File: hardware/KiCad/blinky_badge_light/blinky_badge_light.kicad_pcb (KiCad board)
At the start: 4 copper layers, 108.6 x 87.8 mm, 120 parts, among them Q1 N-Channel MOSFET, Q2 Q_PMOS_GSD, Q3 N-Channel MOSFET, SW1 TS-1187A-B-A-B, U1 ESP32-S3-WROOM-1, U2 TP4056, U3 AP2112K-3.3, U4 MT3608, U5 CP2102N-Axx-xQFN24, U6 SN74LVC1T45DBV

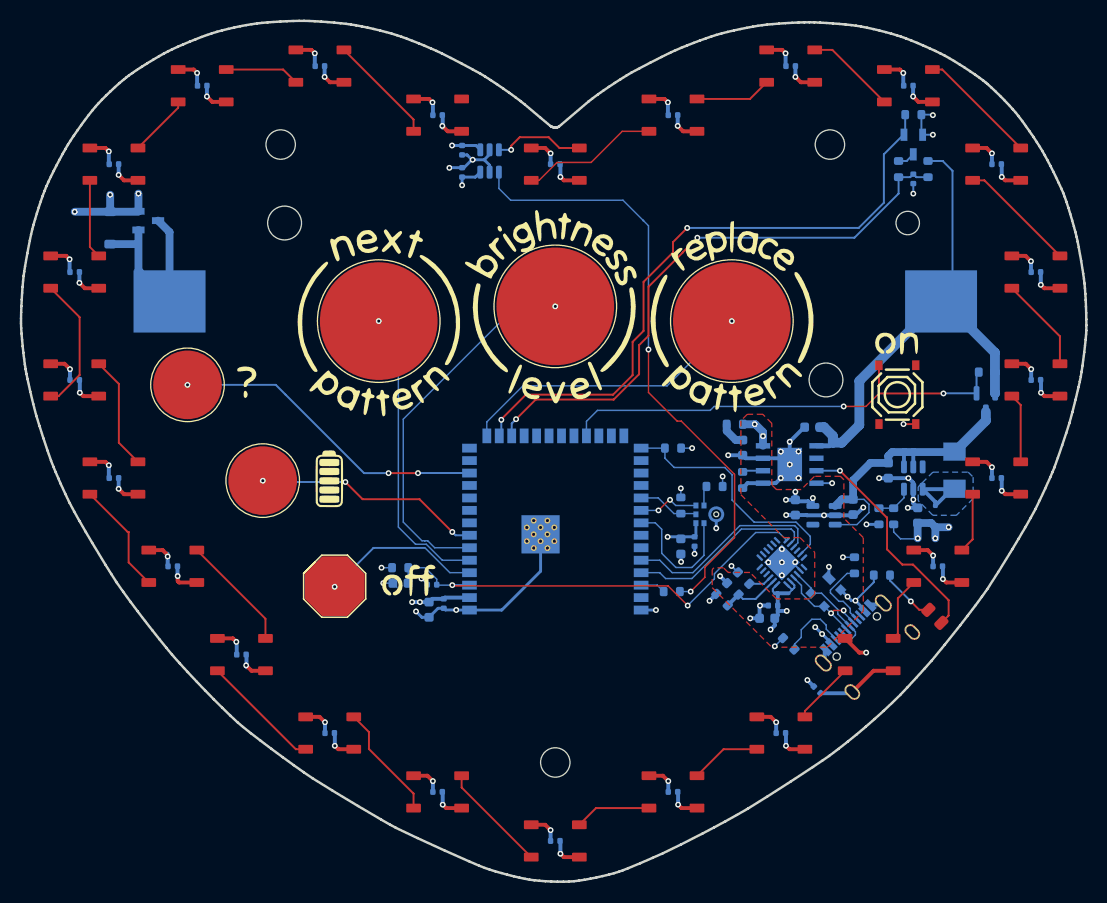
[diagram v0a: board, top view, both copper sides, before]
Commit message: hanger ring
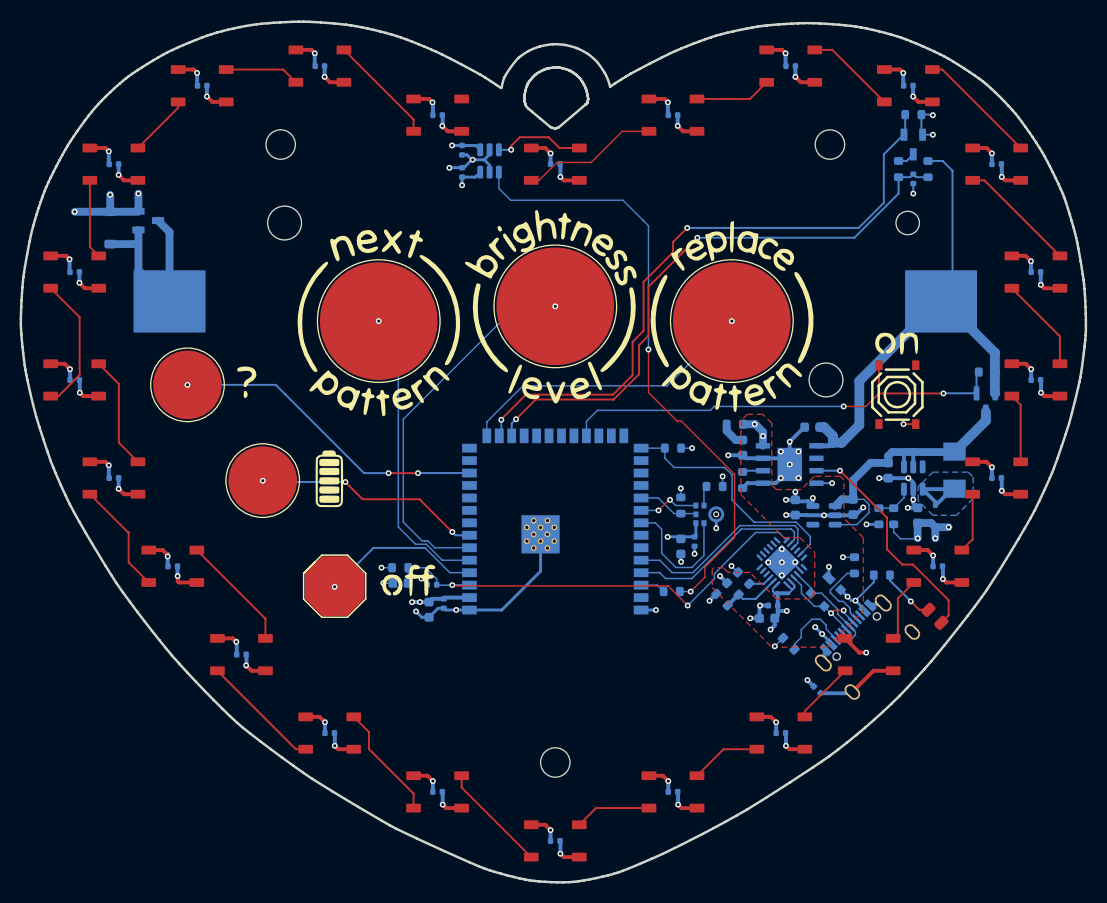
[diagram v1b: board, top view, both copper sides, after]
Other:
- board size 108.6 x 87.8 mm -> 108.6 x 87.7 mm
